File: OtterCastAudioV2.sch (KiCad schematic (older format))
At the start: 26 parts

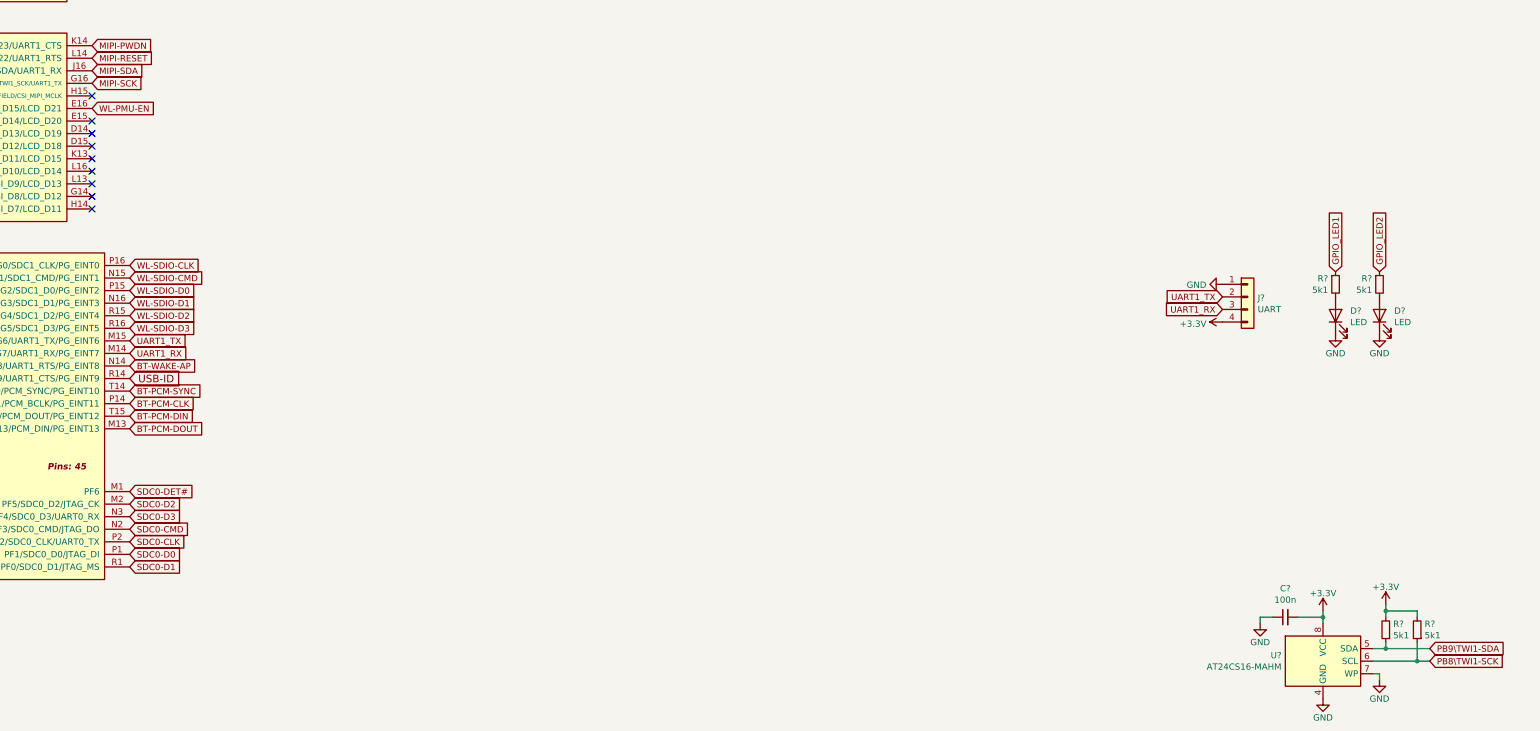
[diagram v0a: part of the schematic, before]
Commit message: update
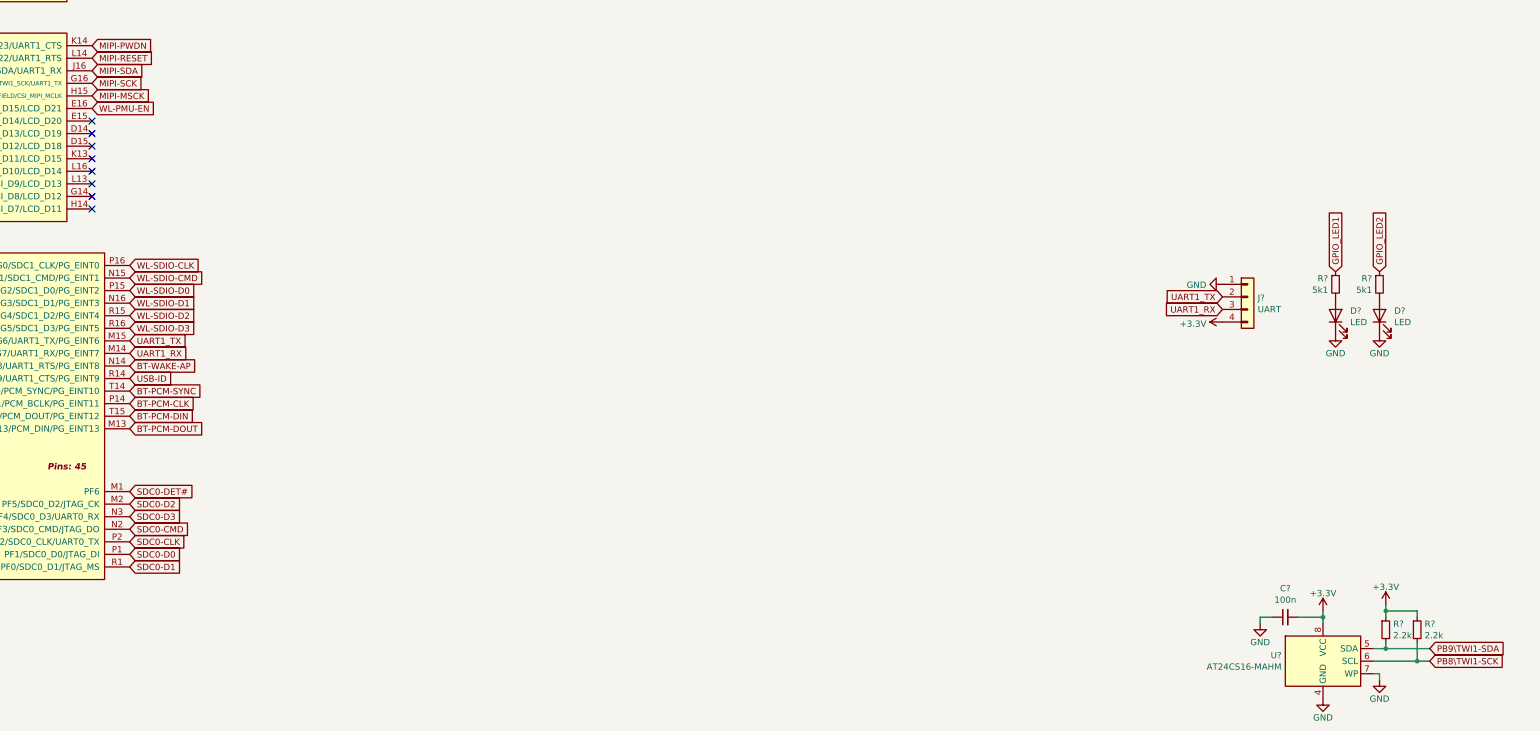
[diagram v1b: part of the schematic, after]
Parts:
- removed R? (x2): 5k1, otter:C_0402, symbol Device:R_Small
- added R? (x2): 2.2k, otter:C_0402, symbol Device:R_Small
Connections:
- net +3V3: now also R?.1, R?.1
- net PB8\TWI1-SCK: now also R?.2
- net PB9\TWI1-SDA: now also R?.2
- net MIPI-MSCK: now reaches U?.H15 (PE20/CSI_FIELD/CSI_MIPI_MCLK)
- no-connect marks 52 -> 51
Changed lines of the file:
@@
 Comment4 ""
 $EndDescr
-Text GLabel 4650 5200 2    60   Input ~ 0
-USB-ID
 $Comp
 L S3-OLinuXino_Rev_A:+3.3V #PWR032
@@
 	1    0    0    -1
 $EndComp
-NoConn ~ 4350 2950
 NoConn ~ 4350 3150
 NoConn ~ 4350 3250
@@
 	1    0    0    -1
 $EndComp
-$Comp
-L otter:AllWinner-S3(FBGA-234) U?
-U 3 1 67AFCAD8
-P 3050 3150
-F 0 "U?" H 3050 4015 50  0000 C CNN
-F 1 "AllWinner-S3(FBGA-234)" H 3050 3924 50  0000 C CNN
-F 2 "OLIMEX_IC-FP:FBGA-234(Pitch-0.65mm_Pad-0.3mm_11x11x1.08mm)" H 3050 1100 50  0001 C CNN
-F 3 "" H 3250 4850 50  0001 C CNN
-	3    3050 3150
-	1    0    0    -1
-$EndComp
 Text GLabel 1750 1300 0    50   Input ~ 0
 GPIO_LED2
@@
 Wire Wire Line
 	13950 7100 14150 7100
-$Comp
-L Device:R_Small R?
-U 1 1 67CD5CEB
-P 14650 7200
-F 0 "R?" H 14591 7154 50  0000 R CNN
-F 1 "5k1" H 14591 7245 50  0000 R CNN
-F 2 "otter:C_0402" H 14650 7200 50  0001 C CNN
-F 3 "~" H 14650 7200 50  0001 C CNN
-	1    14650 7200
-	-1   0    0    1
-$EndComp
-$Comp
-L Device:R_Small R?
-U 1 1 67CD9C01
-P 14900 7200
-F 0 "R?" H 14841 7154 50  0000 R CNN
-F 1 "5k1" H 14841 7245 50  0000 R CNN
-F 2 "otter:C_0402" H 14900 7200 50  0001 C CNN
-F 3 "~" H 14900 7200 50  0001 C CNN
-	1    14900 7200
-	-1   0    0    1
-$EndComp
 Wire Wire Line
 	15000 7350 14650 7350
@@
 	14650 7000 14650 7050
 Connection ~ 14650 7050
+Text GLabel 4650 5200 2    50   Input ~ 0
+USB-ID
+Text GLabel 4350 2950 2    50   Input ~ 0
+MIPI-MSCK
+$Comp
+L otter:AllWinner-S3(FBGA-234) U?
+U 3 1 67AFCAD8
+P 3050 3150
+F 0 "U?" H 3050 4015 50  0000 C CNN
+F 1 "AllWinner-S3(FBGA-234)" H 3050 3924 50  0000 C CNN
+F 2 "OLIMEX_IC-FP:FBGA-234(Pitch-0.65mm_Pad-0.3mm_11x11x1.08mm)" H 3050 1100 50  0001 C CNN
+F 3 "" H 3250 4850 50  0001 C CNN
+	3    3050 3150
+	1    0    0    -1
+$EndComp
+$Comp
+L Device:R_Small R?
+U 1 1 5FFC46C5
+P 14650 7200
+AR Path="/5FFC46C5" Ref="R?"  Part="1"
+AR Path="/602ACDF9/5FFC46C5" Ref="R?"  Part="1"
+F 0 "R?" H 14709 7246 50  0000 L CNN
+F 1 "2.2k" H 14709 7155 50  0000 L CNN
+F 2 "otter:C_0402" H 14650 7200 50  0001 C CNN
+F 3 "~" H 14650 7200 50  0001 C CNN
+	1    14650 7200
+	1    0    0    -1
+$EndComp
+$Comp
+L Device:R_Small R?
+U 1 1 5FFC572E
+P 14900 7200
+AR Path="/5FFC572E" Ref="R?"  Part="1"
+AR Path="/602ACDF9/5FFC572E" Ref="R?"  Part="1"
+F 0 "R?" H 14959 7246 50  0000 L CNN
+F 1 "2.2k" H 14959 7155 50  0000 L CNN
+F 2 "otter:C_0402" H 14900 7200 50  0001 C CNN
+F 3 "~" H 14900 7200 50  0001 C CNN
+	1    14900 7200
+	1    0    0    -1
+$EndComp
 $EndSCHEMATC

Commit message: update
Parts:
- gave numbers to parts that had none: 24
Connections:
- net labels added: MIC-DET
- net labels removed: HP(MIC)-DET
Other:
- moved on the sheet: C1, C2, C3, C4, D1, D2, FB1, J1, J2, R1, R10, R11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

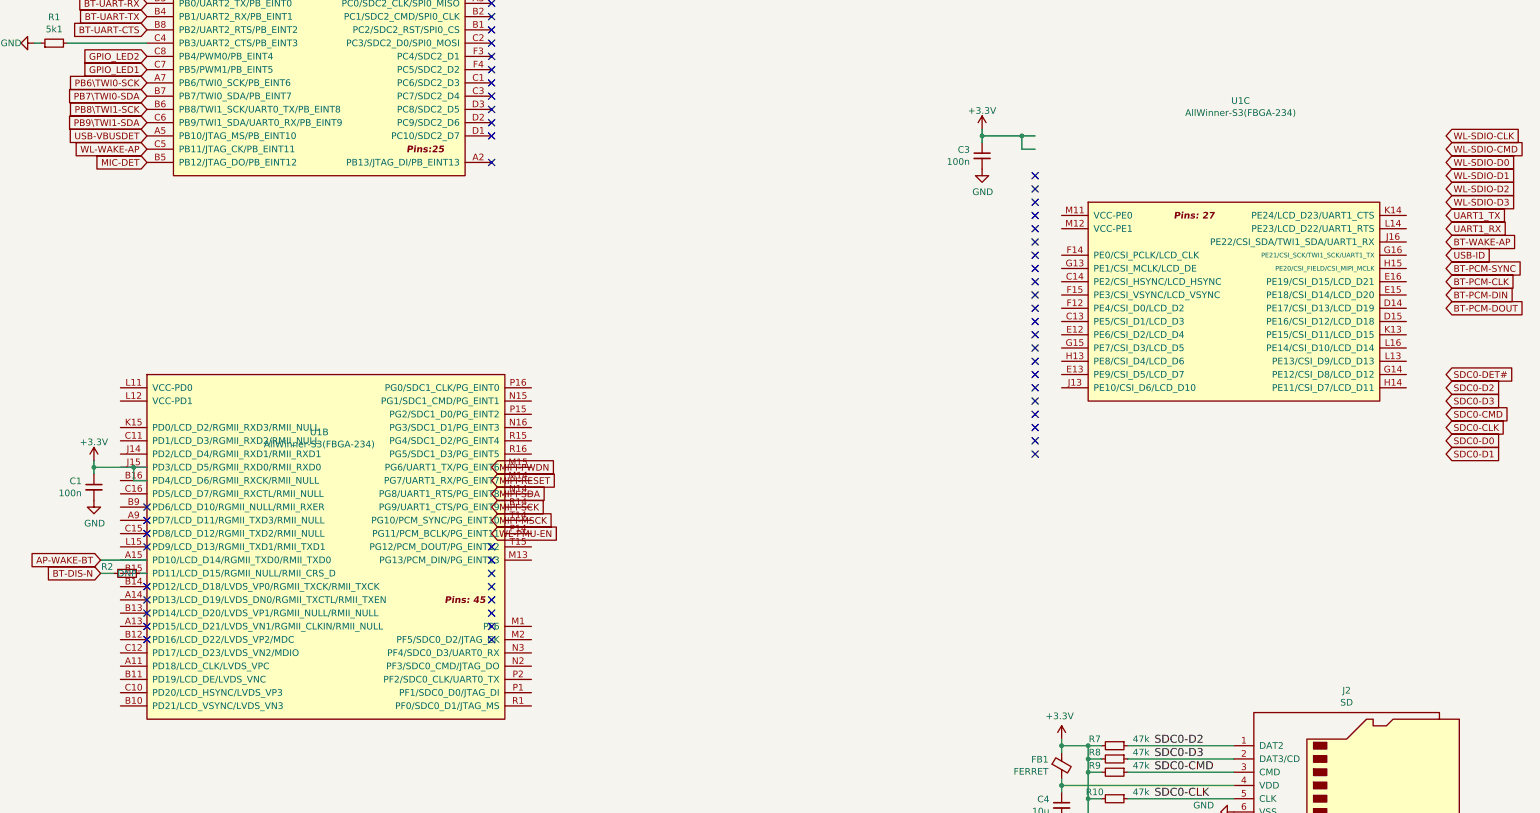
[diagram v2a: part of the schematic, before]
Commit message: update
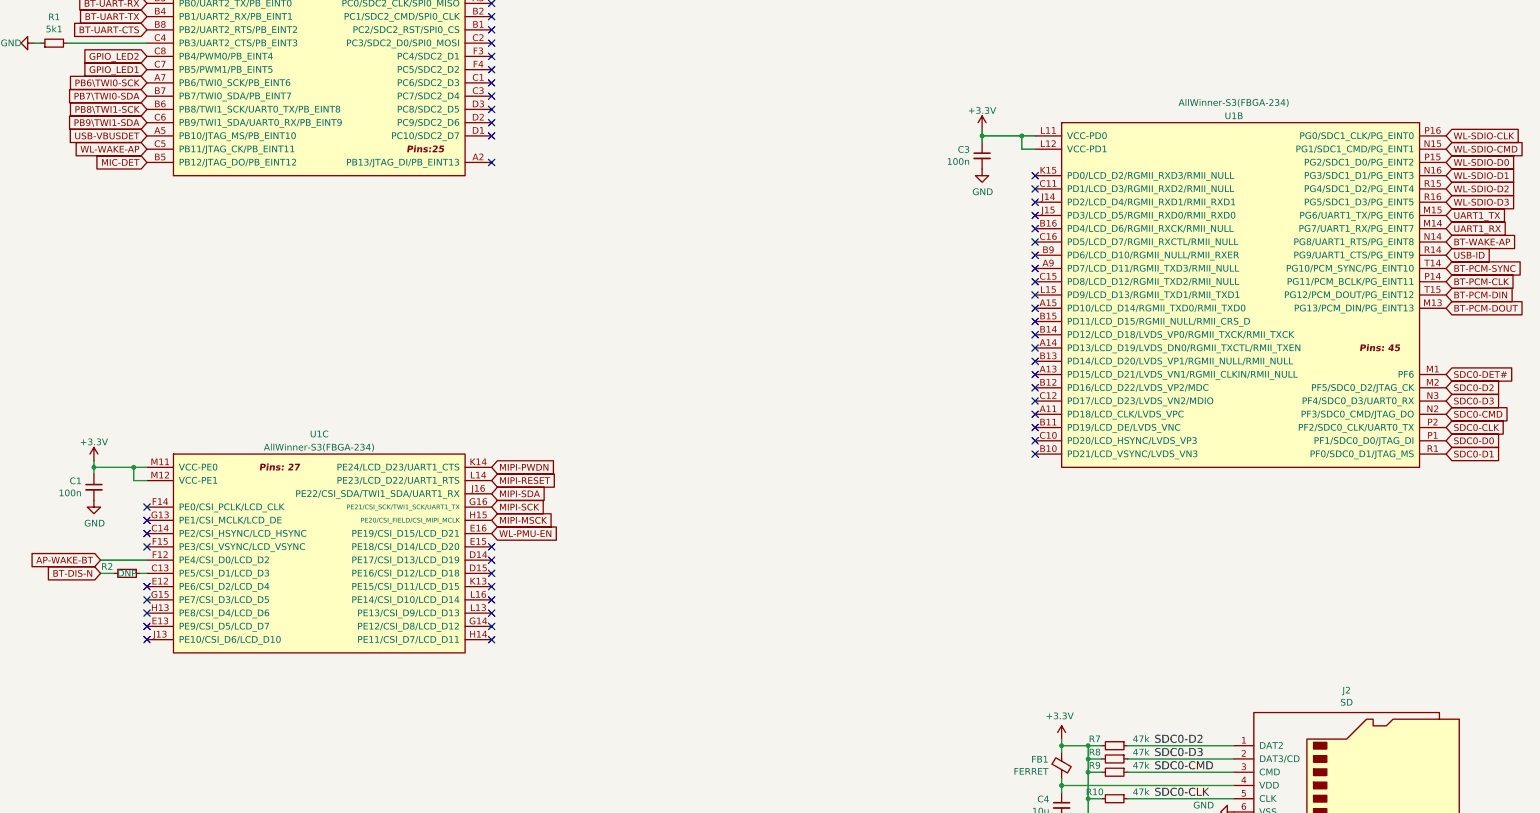
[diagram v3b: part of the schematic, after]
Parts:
- D1, D2: footprint (none) -> otter:LED_0603_1608Metric
- J1: footprint (none) -> Connector_PinHeader_2.00mm:PinHeader_1x04_P2.00mm_Vertical
- J2: footprint (none) -> Connector_Card:microSD_HC_Hirose_DM3D-SF
- U1: footprint OLIMEX_IC-FP:FBGA-234(Pitch-0.65mm_Pad-0.3mm_11x11x1.08mm) -> otter:FBGA-234(Pitch-0.65mm_Pad-0.3mm_11x11x1.08mm)
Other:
- moved on the sheet: U1B, U1C
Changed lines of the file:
@@
 F 0 "J2" H 13200 9117 50  0000 C CNN
 F 1 "SD" H 13200 9026 50  0000 C CNN
-F 2 "" H 15300 9000 50  0001 C CNN
+F 2 "Connector_Card:microSD_HC_Hirose_DM3D-SF" H 15300 9000 50  0001 C CNN
 F 3 "https://www.hirose.com/product/en/download_file/key_name/DM3/category/Catalog/doc_file_id/49662/?file_category_id=4&item_id=195&is_series=1" H 13250 8400 50  0001 C CNN
 	1    13250 8300
@@
 F 0 "J1" H 7480 10392 50  0000 L CNN
 F 1 "UART" H 7480 10301 50  0000 L CNN
-F 2 "" H 7400 10400 50  0001 C CNN
+F 2 "Connector_PinHeader_2.00mm:PinHeader_1x04_P2.00mm_Vertical" H 7400 10400 50  0001 C CNN
 F 3 "~" H 7400 10400 50  0001 C CNN
 	1    7400 10400
@@
 F 0 "D1" V 8139 10433 50  0000 R CNN
 F 1 "LED" V 8048 10433 50  0000 R CNN
-F 2 "" H 8100 10550 50  0001 C CNN
+F 2 "otter:LED_0603_1608Metric" H 8100 10550 50  0001 C CNN
 F 3 "~" H 8100 10550 50  0001 C CNN
 	1    8100 10550
@@
 Wire Wire Line
 	4100 6600 4150 6600
-Wire Wire Line
-	4150 6500 3800 6500
 NoConn ~ 4150 6100
 NoConn ~ 4150 6200
@@
 	1    0    0    -1
 $EndComp
-Wire Wire Line
-	4050 5800 3750 5800
 Connection ~ 4050 5800
 Connection ~ 3750 5800
@@
 F 0 "U1" H 5450 3765 50  0000 C CNN
 F 1 "AllWinner-S3(FBGA-234)" H 5450 3674 50  0000 C CNN
-F 2 "OLIMEX_IC-FP:FBGA-234(Pitch-0.65mm_Pad-0.3mm_11x11x1.08mm)" H 5450 850 50  0001 C CNN
+F 2 "otter:FBGA-234(Pitch-0.65mm_Pad-0.3mm_11x11x1.08mm)" H 5450 850 50  0001 C CNN
 F 3 "" H 5650 4600 50  0001 C CNN
 	1    5450 2900
@@
 L otter:AllWinner-S3(FBGA-234) U1
 U 3 1 67AF4AB4
-P 12350 4500
-F 0 "U1" H 12400 5965 50  0000 C CNN
-F 1 "AllWinner-S3(FBGA-234)" H 12400 5874 50  0000 C CNN
-F 2 "OLIMEX_IC-FP:FBGA-234(Pitch-0.65mm_Pad-0.3mm_11x11x1.08mm)" H 12350 2450 50  0001 C CNN
-F 3 "" H 12550 6200 50  0001 C CNN
-	3    12350 4500
+P 5450 6400
+F 0 "U1" H 5450 7250 50  0000 C CNN
+F 1 "AllWinner-S3(FBGA-234)" H 5450 7150 50  0000 C CNN
+F 2 "otter:FBGA-234(Pitch-0.65mm_Pad-0.3mm_11x11x1.08mm)" H 5450 4350 50  0001 C CNN
+F 3 "" H 5650 8100 50  0001 C CNN
+	3    5450 6400
 	1    0    0    -1
 $EndComp
@@
 F 0 "D2" V 8489 10433 50  0000 R CNN
 F 1 "LED" V 8398 10433 50  0000 R CNN
-F 2 "" H 8450 10550 50  0001 C CNN
+F 2 "otter:LED_0603_1608Metric" H 8450 10550 50  0001 C CNN
 F 3 "~" H 8450 10550 50  0001 C CNN
 	1    8450 10550
@@
 L otter:AllWinner-S3(FBGA-234) U1
 U 2 1 67AFCAD8
-P 5450 6400
-F 0 "U1" H 5450 7265 50  0000 C CNN
-F 1 "AllWinner-S3(FBGA-234)" H 5450 7174 50  0000 C CNN
-F 2 "OLIMEX_IC-FP:FBGA-234(Pitch-0.65mm_Pad-0.3mm_11x11x1.08mm)" H 5450 4350 50  0001 C CNN
-F 3 "" H 5650 8100 50  0001 C CNN
-	2    5450 6400
+P 12350 4500
+F 0 "U1" H 12350 5850 50  0000 C CNN
+F 1 "AllWinner-S3(FBGA-234)" H 12350 5950 50  0000 C CNN
+F 2 "otter:FBGA-234(Pitch-0.65mm_Pad-0.3mm_11x11x1.08mm)" H 12350 2450 50  0001 C CNN
+F 3 "" H 12550 6200 50  0001 C CNN
+	2    12350 4500
 	1    0    0    -1
 $EndComp
@@
 	1    0    0    -1
 $EndComp
+Wire Wire Line
+	3800 6500 4150 6500
+Wire Wire Line
+	3750 5800 4050 5800
 $EndSCHEMATC
